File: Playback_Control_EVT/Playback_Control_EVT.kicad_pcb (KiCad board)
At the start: 2 copper layers, 66 x 63.5 mm, 24 parts, among them J1 Conn_01x05_Pin, J2 Conn_01x04_Pin, J3 Conn_01x03_Pin, J4 Conn_01x03_Pin, J5 Conn_01x03_Pin, Q1 BC547, Q2 BC547, Q3 BC547, U1 STM32L432KCUx, U2 J104D2C3VDC.20S, U3 J104D2C3VDC.20S, U4 J104D2C3VDC.20S

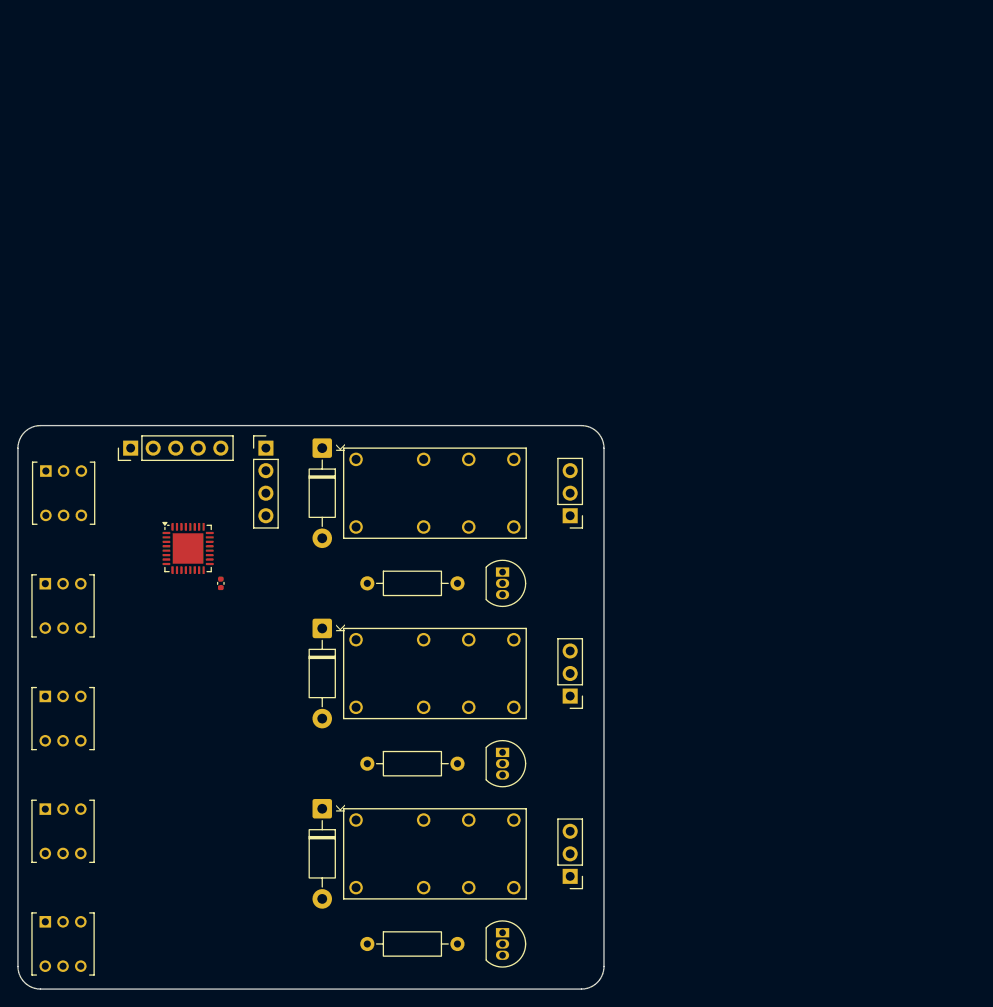
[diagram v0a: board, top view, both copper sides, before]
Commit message: Order
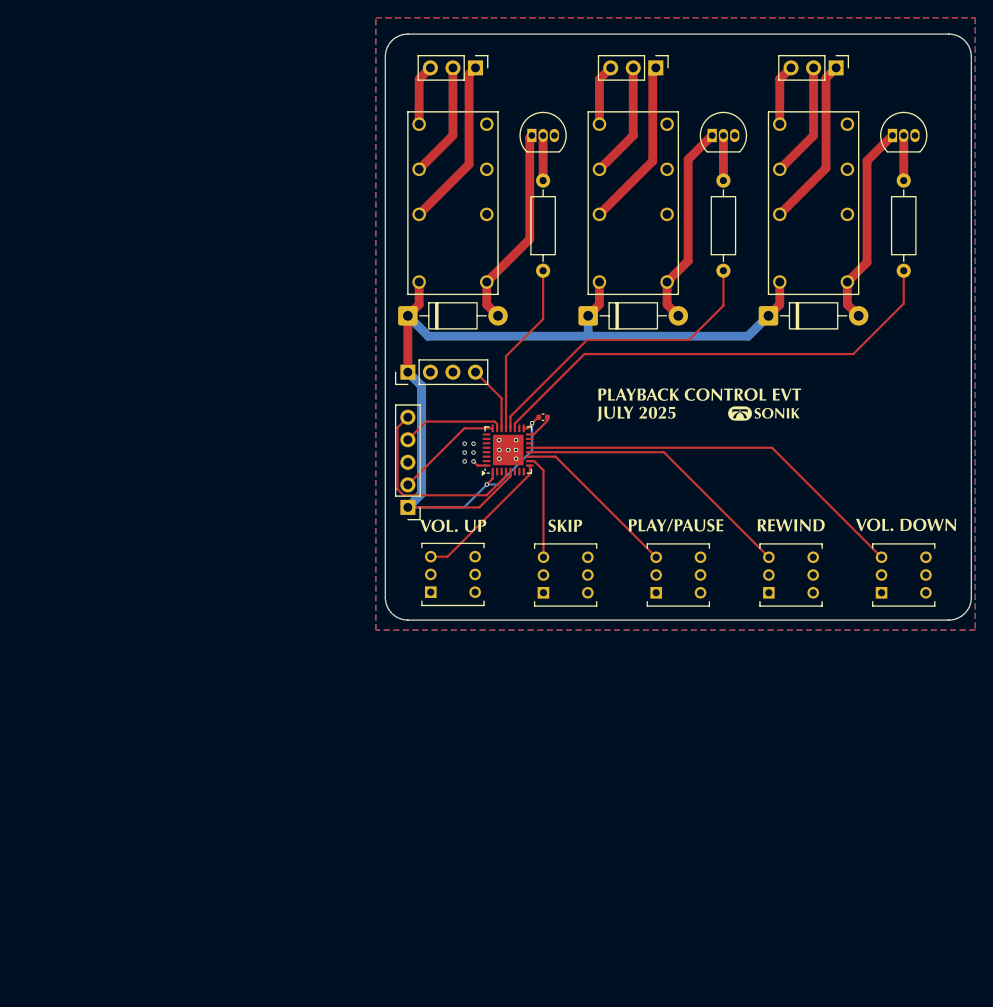
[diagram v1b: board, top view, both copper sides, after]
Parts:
- added G***: LOGO, LOGO, F.Cu at (155.2, 97.7)
- added G***: LOGO, LOGO, F.Cu at (148.0, 96.7)
- added G***: LOGO, LOGO, F.Cu at (122.1, 110.4)
- added G***: LOGO, LOGO, F.Cu at (145.5, 110.4)
- added G***: LOGO, LOGO, F.Cu at (160.0, 110.3)
- added G***: LOGO, LOGO, F.Cu at (136.5, 110.4)
- added G***: LOGO, LOGO, F.Cu at (171.2, 110.3)
- moved S5 103.5 mm to (170.9, 115.9), turned to 90 degrees
- moved Q3 100.0 mm to (169.7, 66.4), turned to 0 degrees
- moved R3 97.0 mm to (170.9, 81.6), turned to 90 degrees
- moved J5 95.9 mm to (163.3, 58.8), turned to -90 degrees
- moved U4 87.9 mm to (164.6, 82.9), turned to 180 degrees
- moved S4 87.0 mm to (158.2, 115.9), turned to 90 degrees
- moved D3 74.9 mm to (155.7, 86.7), turned to 0 degrees
- moved Q2 73.4 mm to (149.3, 66.4), turned to 0 degrees
- moved J4 71.4 mm to (143.0, 58.8), turned to -90 degrees
- moved S3 71.2 mm to (145.5, 115.9), turned to 90 degrees
- moved R2 68.5 mm to (150.6, 81.6), turned to 90 degrees
- moved U3 59.4 mm to (144.3, 82.9), turned to 180 degrees
- moved S2 56.7 mm to (132.8, 115.9), turned to 90 degrees
- moved J3 51.6 mm to (122.7, 58.8), turned to -90 degrees
- moved Q1 49.3 mm to (129.0, 66.4), turned to 0 degrees
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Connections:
- R1 pad 1: Net-(U1-PA12) -> Net-(U1-PA11)
- R2 pad 1: Net-(U1-PA11) -> Net-(U1-PA10)
- R3 pad 1: Net-(U1-PA10) -> Net-(U1-PA9)
- U1 pad 14: /~{EN} -> unconnected-(U1-PB0-Pad14)
- U1 pad 19: unconnected-(U1-PA9-Pad19) -> Net-(U1-PA9)
- U1 pad 22: Net-(U1-PA12) -> /~{EN}
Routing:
- net VDD: track 0.00 -> 118.0 mm, vias 0 -> 2
- net Net-(U1-PA9): track 0.00 -> 53.7 mm
- net /Vol-: track 0.00 -> 44.7 mm
- net Net-(U1-PA10): track 0.00 -> 34.4 mm
- net /Rwd: track 0.00 -> 31.8 mm
- net Net-(D3-A): track 0.00 -> 23.0 mm
- net Net-(D2-A): track 0.00 -> 23.0 mm
- net Net-(D1-A): track 0.00 -> 23.0 mm
- net /NRST: track 0.00 -> 22.5 mm
- net Net-(U1-PA11): track 0.00 -> 19.5 mm
- net Net-(J3-Pin_1): track 0.00 -> 19.1 mm
- net Net-(J5-Pin_1): track 0.00 -> 19.1 mm
- net Net-(J4-Pin_1): track 0.00 -> 19.1 mm
- net /Play: track 0.00 -> 18.9 mm
- net /Vol+: track 0.00 -> 16.0 mm
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- added copper zone on B.Cu, net GND
- added copper zone on F.Cu, net GND
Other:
- board size 66 x 63.5 mm -> 66 x 66 mm
